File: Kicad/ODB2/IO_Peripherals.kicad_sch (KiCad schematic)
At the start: 22 parts, among them J5 RFM_Conn_Coaxial, U10 W25Q512JVEIQ

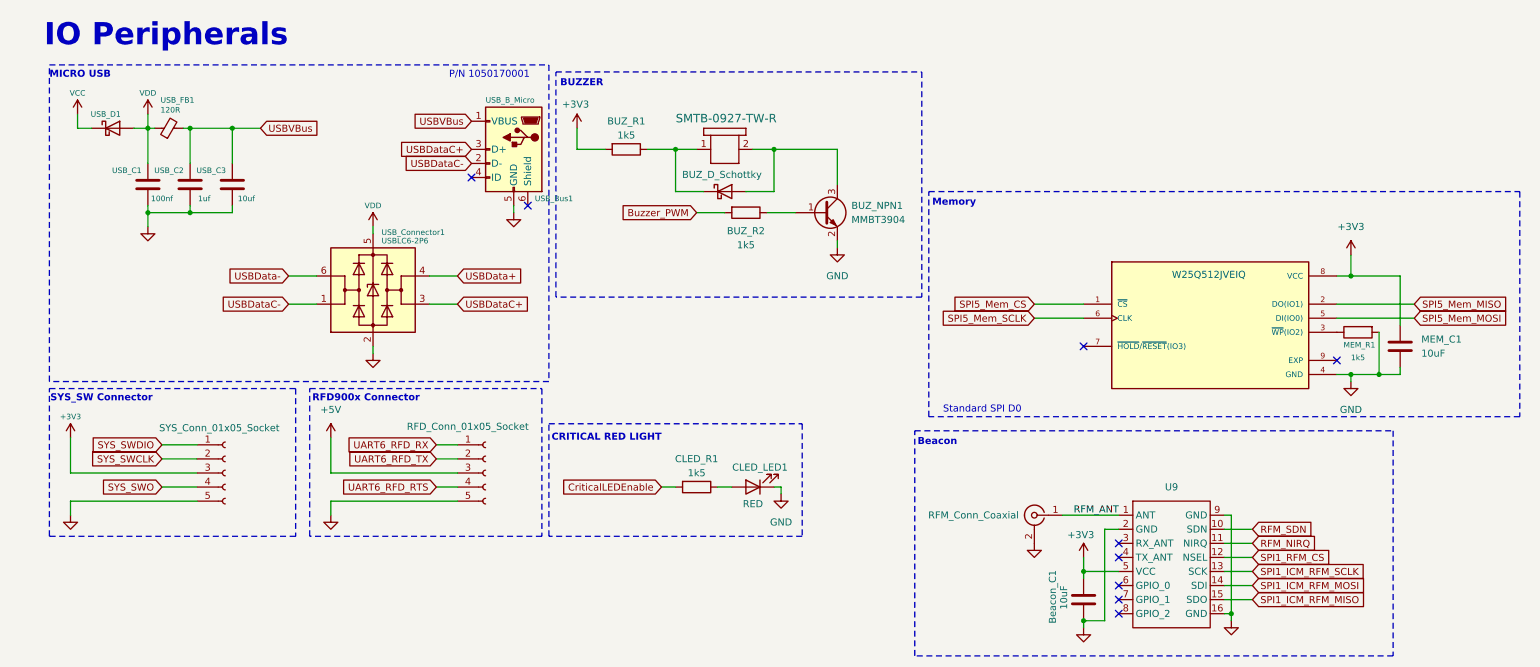
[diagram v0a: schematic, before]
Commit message: Fix somes issue
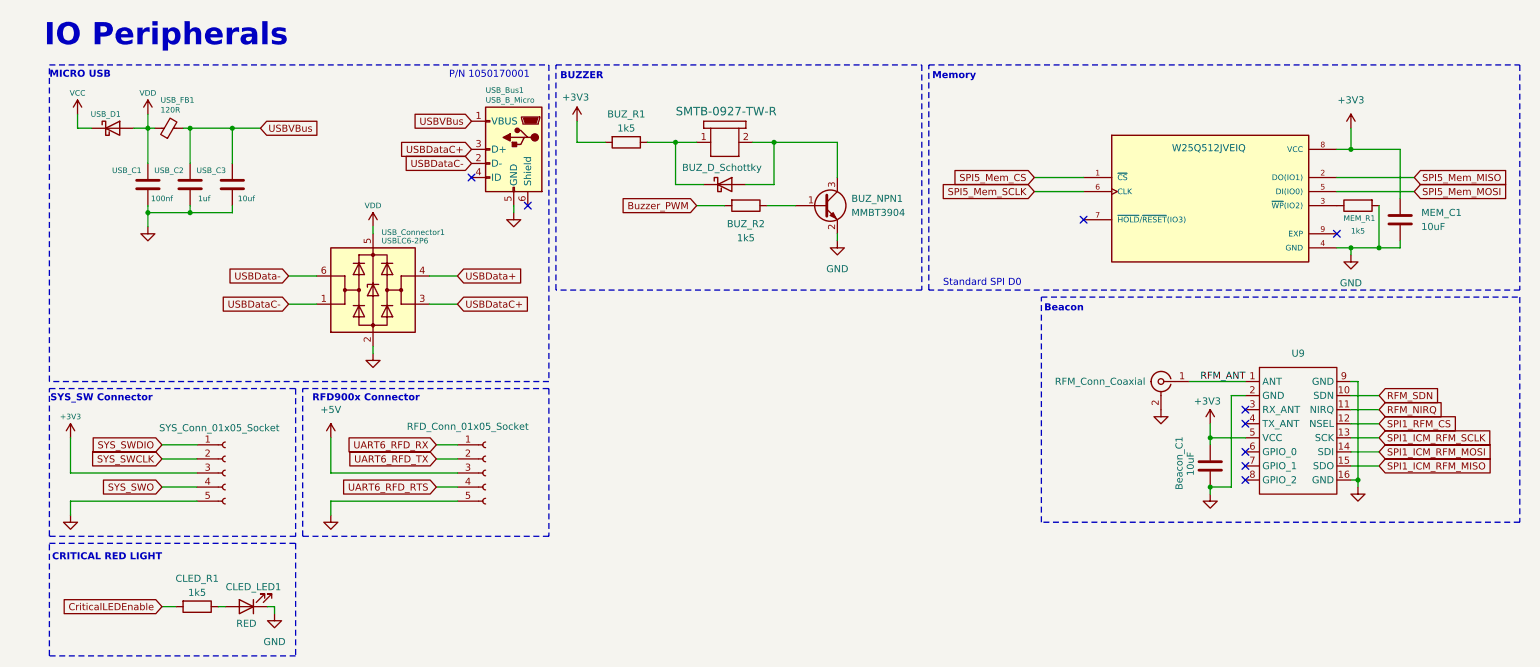
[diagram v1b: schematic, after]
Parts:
- BUZ_R1, BUZ_R2, CLED_R1, MEM_R1: footprint Resistor_SMD:R_0805_2012Metric -> Resistor_SMD:R_0603_1608Metric
- Beacon_C1, MEM_C1, USB_C1, USB_C2, USB_C3: footprint Capacitor_SMD:C_0805_2012Metric -> Capacitor_SMD:C_0603_1608Metric
- CLED_LED1: footprint LED_SMD:LED_0805_2012Metric -> LED_SMD:LED_0603_1608Metric
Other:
- moved on the sheet: BUZ_NPN1, BUZ_R1, BUZ_R2, Beacon_C1, CLED_LED1, CLED_R1, MEM_C1, MEM_R1, U9
